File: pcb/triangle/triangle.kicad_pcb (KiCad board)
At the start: 2 copper layers, 56.8 x 65.5 mm, 65 parts, among them J1 Conn_01x03_Male, J2 Conn_01x03_Male

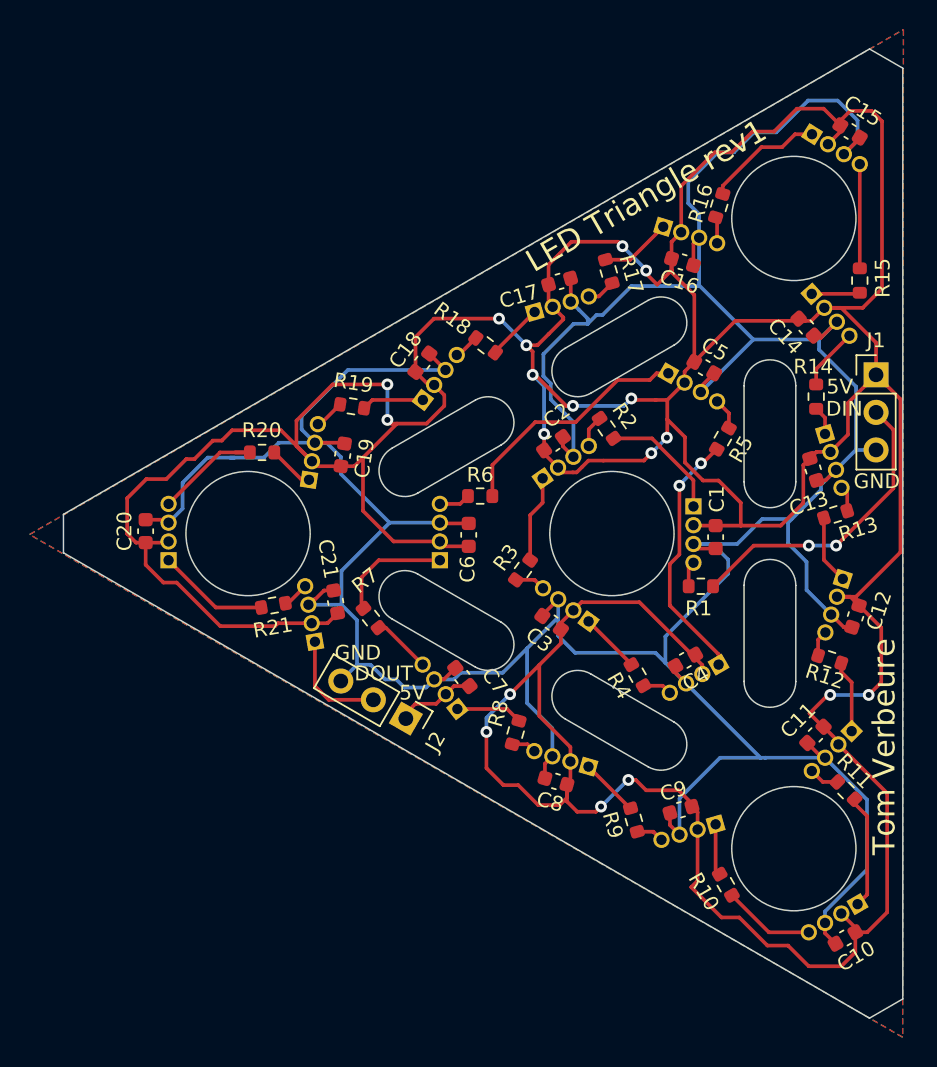
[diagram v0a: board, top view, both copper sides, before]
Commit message: Triangle PCB v2.
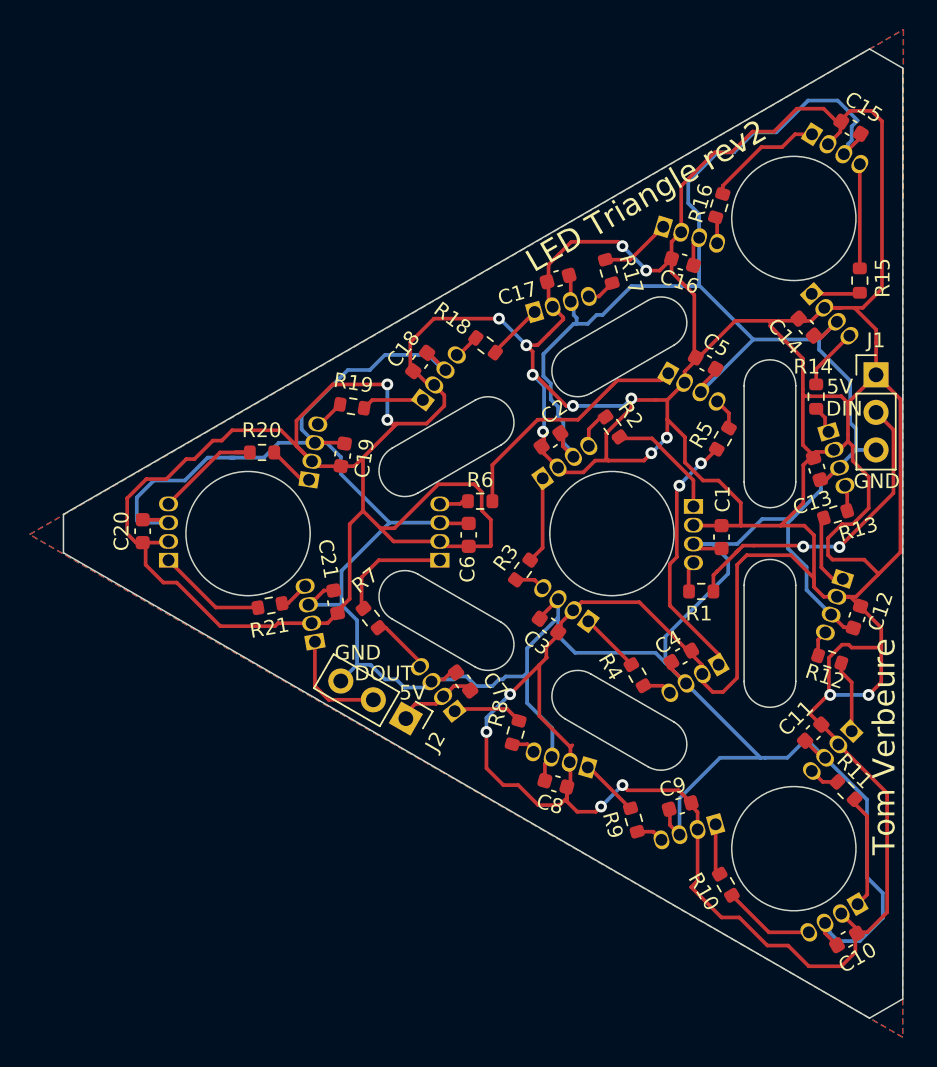
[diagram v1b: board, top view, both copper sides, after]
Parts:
- moved R2 0.41 mm to (142.2, 76.4)
- moved C1 0.40 mm to (149.6, 83.9)
- moved C4 0.39 mm to (146.9, 91.9)
- moved R1 0.35 mm to (148.2, 87.5)
- moved R6 0.35 mm to (133.3, 81.5)
- moved C5 0.32 mm to (148.5, 72.1)
- moved C2 0.31 mm to (138.1, 77.3)
- moved C7 0.30 mm to (132.1, 93.6)
- moved D13 0.28 mm to (157.4, 78.6)
- moved C3 0.26 mm to (137.9, 89.9)
- moved C15 0.26 mm to (158.4, 56.2)
- moved C13 0.25 mm to (156.1, 79.2)
- moved C9 0.25 mm to (146.8, 102.1)
- moved D7 0.24 mm to (130.4, 94.1)
- moved R21 0.23 mm to (119.1, 88.5)
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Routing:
- net +5V: track 364.6 -> 448.5 mm
- net GND: track 266.2 -> 276.0 mm
- net /DIN: track 20.6 -> 21.8 mm
- net Net-(D12-Pad1): track 4.65 -> 5.19 mm
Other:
- board text added: "LED Triangle rev2"
- board text removed: "LED Triangle rev1"
